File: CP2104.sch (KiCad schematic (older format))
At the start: 8 parts, among them J7 USB_B_Mini, U4 CP2104

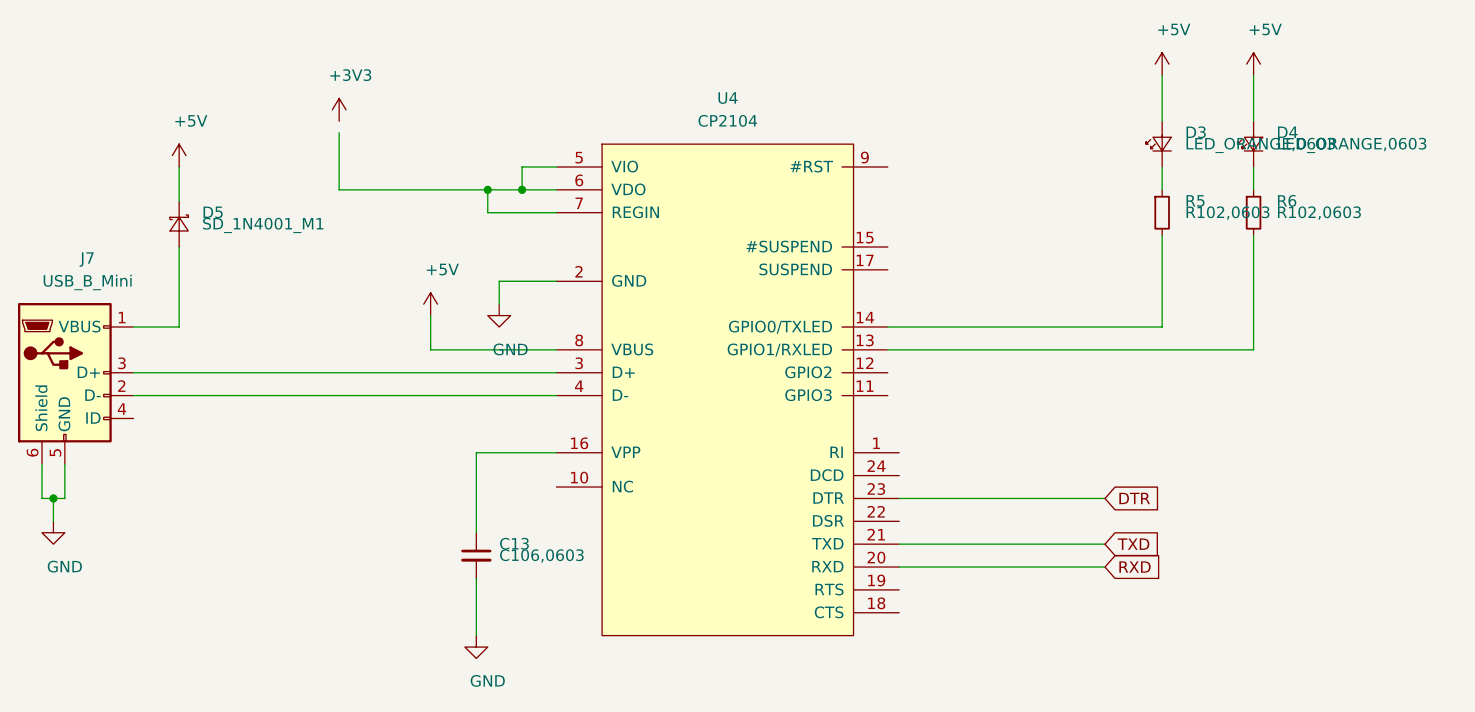
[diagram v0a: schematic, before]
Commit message: update,
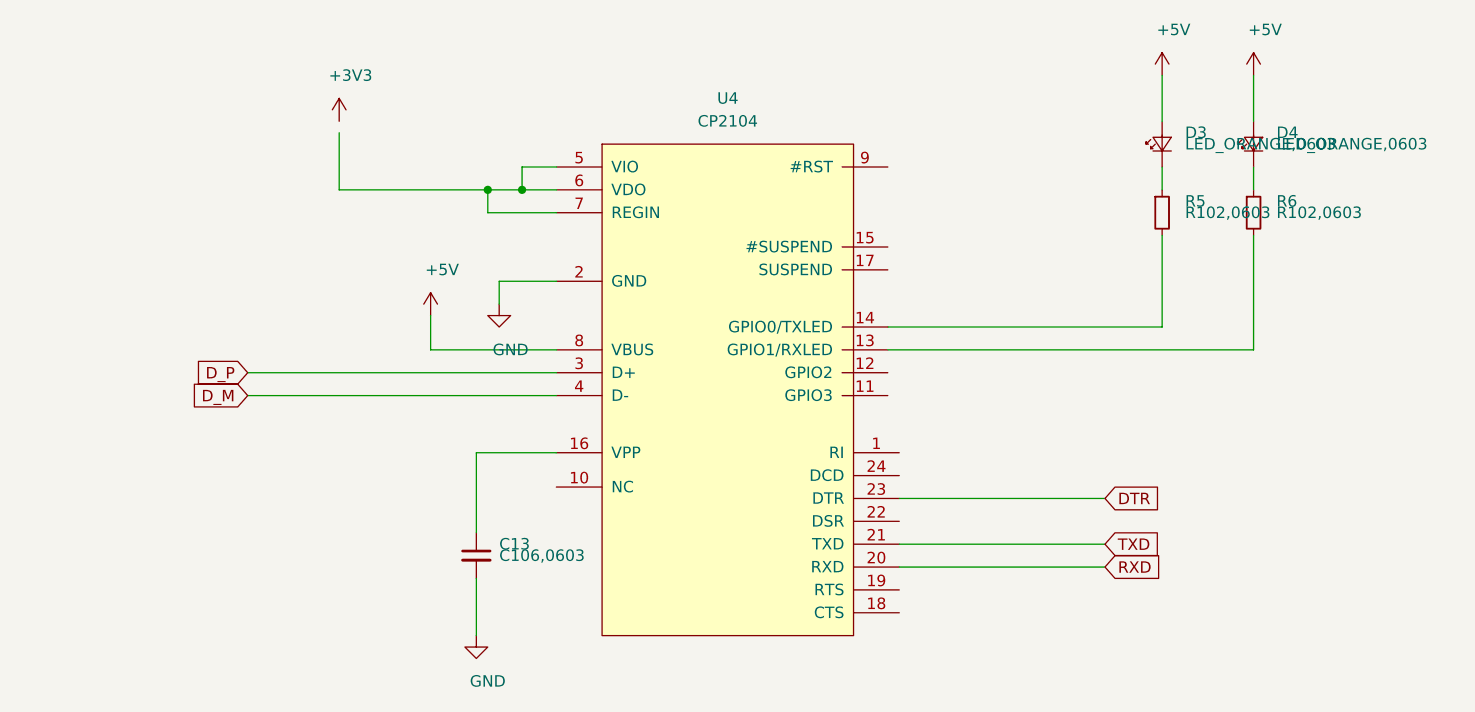
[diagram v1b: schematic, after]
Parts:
- removed D5: SD_1N4001_M1, w_smd_diode:do214ac, symbol taobao-sd:SD_1N4001_M1
- removed J7: USB_B_Mini, Connector_USB:USB_Micro-B_Amphenol_10103594-0001LF_Horizontal, symbol Connector:USB_B_Mini
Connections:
- net labels added: D_M, D_P
- wire segments 36 -> 28
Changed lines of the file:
@@
 $EndDescr
-$Comp
-L Connector:USB_B_Mini J7
-U 1 1 5C0C4517
-P 3250 3200
-F 0 "J7" H 3350 3700 50  0000 C CNN
-F 1 "USB_B_Mini" H 3350 3600 50  0000 C CNN
-F 2 "Connector_USB:USB_Micro-B_Amphenol_10103594-0001LF_Horizontal" H 3400 3150 50  0001 C CNN
-F 3 "~" H 3400 3150 50  0001 C CNN
-	1    3250 3200
-	1    0    0    -1
-$EndComp
-Wire Wire Line
-	3550 3200 5400 3200
-Wire Wire Line
-	3550 3300 5400 3300
-$Comp
-L power:GND #PWR0128
-U 1 1 5C0C45BE
-P 3200 3850
-F 0 "#PWR0128" H 3200 3600 50  0001 C CNN
-F 1 "GND" H 3250 3650 50  0000 C CNN
-F 2 "" H 3200 3850 50  0001 C CNN
-F 3 "" H 3200 3850 50  0001 C CNN
-	1    3200 3850
-	1    0    0    -1
-$EndComp
-Wire Wire Line
-	3150 3600 3150 3750
-Wire Wire Line
-	3150 3750 3200 3750
-Wire Wire Line
-	3200 3750 3200 3850
-Wire Wire Line
-	3250 3600 3250 3750
-Wire Wire Line
-	3250 3750 3200 3750
-Connection ~ 3200 3750
-$Comp
-L power:+5V #PWR0129
-U 1 1 5C0C464F
-P 3750 2300
-F 0 "#PWR0129" H 3750 2150 50  0001 C CNN
-F 1 "+5V" H 3800 2500 50  0000 C CNN
-F 2 "" H 3750 2300 50  0001 C CNN
-F 3 "" H 3750 2300 50  0001 C CNN
-	1    3750 2300
-	1    0    0    -1
-$EndComp
-Wire Wire Line
-	3750 2300 3750 2450
-Wire Wire Line
-	3750 2650 3750 3000
-Wire Wire Line
-	3750 3000 3550 3000
 $Comp
 L power:+3V3 #PWR0130
@@
 	1    0    0    -1
 $EndComp
-$Comp
-L taobao-sd:SD_1N4001_M1 D5
-U 1 1 5C0DACA6
-P 3750 2550
-F 0 "D5" V 3700 2650 50  0000 L CNN
-F 1 "SD_1N4001_M1" V 3750 2650 50  0000 L CNN
-F 2 "w_smd_diode:do214ac" V 3750 2550 50  0001 C CNN
-F 3 "~" V 3750 2550 50  0001 C CNN
-	1    3750 2550
-	0    1    1    0
-$EndComp
+Text GLabel 4050 3300 0    50   Input ~ 0
+D_M
+Text GLabel 4050 3200 0    50   Input ~ 0
+D_P
+Wire Wire Line
+	4050 3200 5400 3200
+Wire Wire Line
+	4050 3300 5400 3300
 $EndSCHEMATC
